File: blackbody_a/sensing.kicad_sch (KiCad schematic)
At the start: 4 parts, among them U1 LTC4311CSC6-TRPBF

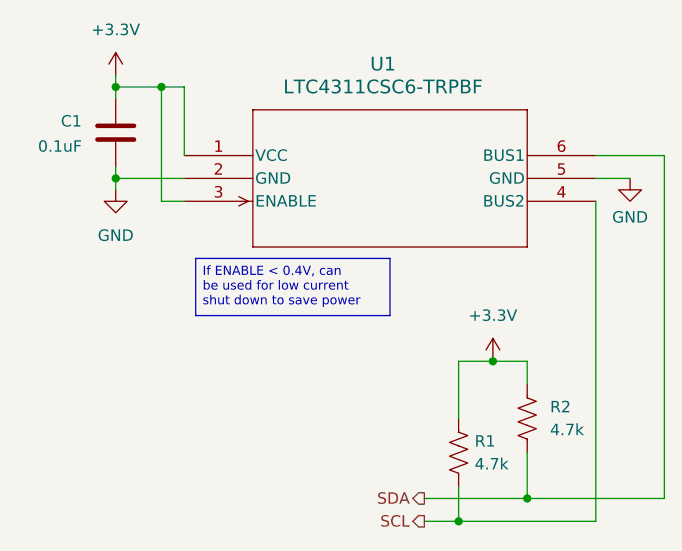
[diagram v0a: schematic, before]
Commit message: layout updates
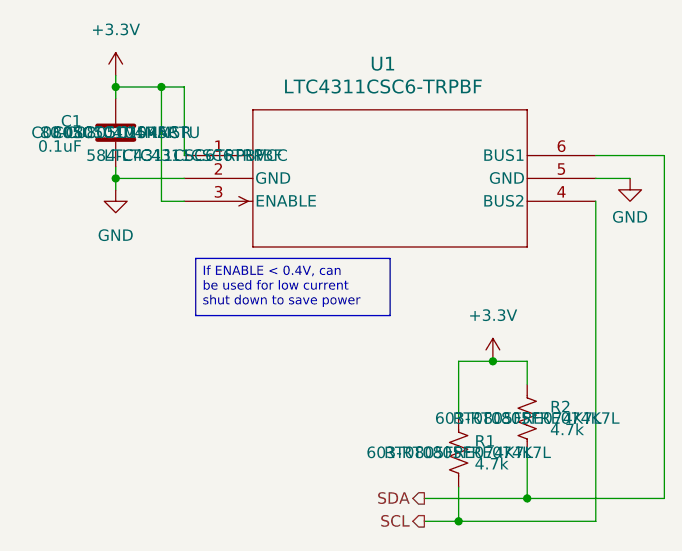
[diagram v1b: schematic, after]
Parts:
- C1: Manufacturer_Part_Number (none) -> C0805C104M5R; Mouser Part Number (none) -> 80-C0805C104M5R; PN (none) -> C0805C104M5RACTU
- R1, R2: Mouser Part Number (none) -> 603-RT0805FRE074K7L; PN (none) -> RT0805FRE074K7L
- U1: Mouser Part Number (none) -> 584-LTC4311CSC6TRPBF; PN (none) -> LTC4311CSC6TRPBF
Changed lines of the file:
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@@
+			)
+		)
+		(property "Mouser Part Number" "603-RT0805FRE074K7L "
+			(at 114.3 92.71 0)
+			(effects
+				(font
+					(size 1.27 1.27)
+				)
+			)
+		)
+		(property "PN" "RT0805FRE074K7L"
+			(at 114.3 92.71 0)
+			(effects
+				(font
+					(size 1.27 1.27)
+				)
 			)
 		)
@@
 			)
 		)
+		(property "Mouser Part Number" "584-LTC4311CSC6TRPBF"
+			(at 83.82 59.69 0)
+			(effects
+				(font
+					(size 1.27 1.27)
+				)
+			)
+		)
+		(property "PN" "LTC4311CSC6TRPBF"
+			(at 83.82 59.69 0)
+			(effects
+				(font
+					(size 1.27 1.27)
+				)
+			)
+		)
 		(pin "1"
 		)
@@
 			)
 		)
+		(property "Mouser Part Number" "603-RT0805FRE074K7L "
+			(at 121.92 88.9 0)
+			(effects
+				(font
+					(size 1.27 1.27)
+				)
+			)
+		)
+		(property "PN" "RT0805FRE074K7L"
+			(at 121.92 88.9 0)
+			(effects
+				(font
+					(size 1.27 1.27)
+				)
+			)
+		)
 		(pin "2"
 		)
@@
 			)
 		)
+		(property "Manufacturer_Part_Number" "C0805C104M5R"
+			(at 76.2 57.15 0)
+			(effects
+				(font
+					(size 1.27 1.27)
+				)
+			)
+		)
+		(property "Mouser Part Number" "80-C0805C104M5R"
+			(at 76.2 57.15 0)
+			(effects
+				(font
+					(size 1.27 1.27)
+				)
+			)
+		)
+		(property "PN" "C0805C104M5RACTU"
+			(at 76.2 57.15 0)
+			(effects
+				(font
+					(size 1.27 1.27)
+				)
+			)
+		)
